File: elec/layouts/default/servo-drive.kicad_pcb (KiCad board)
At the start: 4 copper layers, 42.3 x 42.3 mm, 109 parts

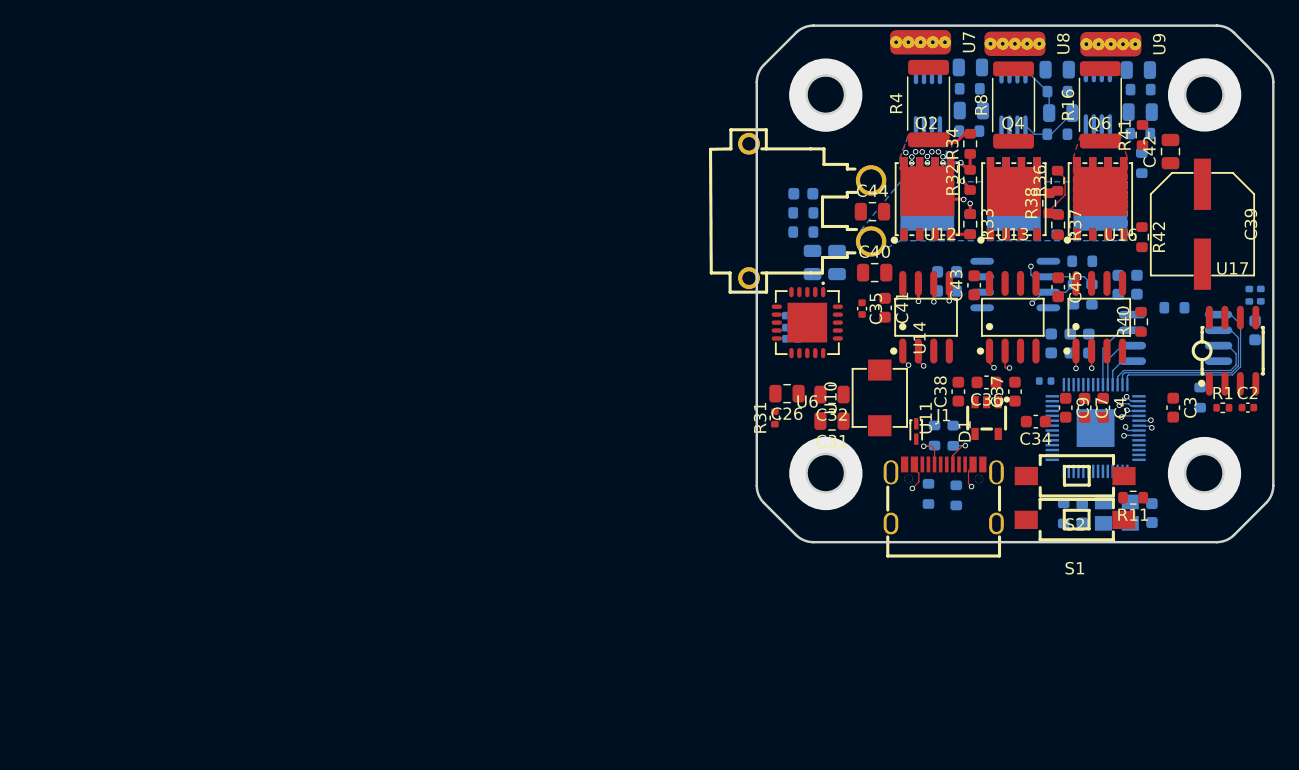
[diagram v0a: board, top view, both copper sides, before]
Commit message: layout complete
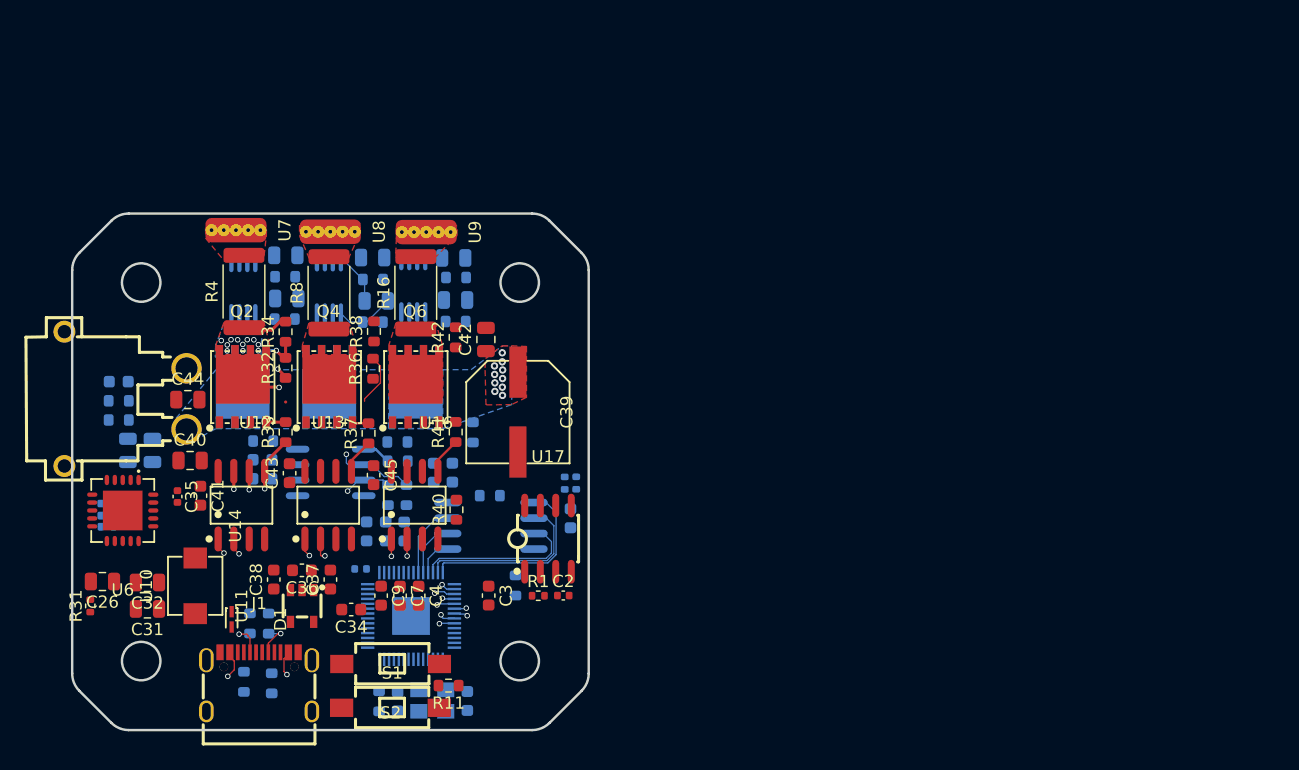
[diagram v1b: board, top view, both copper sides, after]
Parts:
- moved R41 61.3 mm to (162.2, 95.8)
- moved R35 60.6 mm to (146.5, 96.5), turned to 180 degrees
- moved R43 59.1 mm to (163.6, 95.8)
- moved R37 59.0 mm to (155.1, 95.9), turned to 90 degrees
- moved R33 58.6 mm to (148.3, 95.8), turned to 90 degrees
- moved R45 58.5 mm to (158.2, 100.9)
- moved R46 58.5 mm to (156.7, 100.9)
- moved R44 58.4 mm to (157.5, 98.1)
- moved C16 58.1 mm to (148.4, 84.8)
- moved C18 58.1 mm to (155.7, 85.0)
- moved C28 58.1 mm to (137.4, 97.3)
- moved C29 58.1 mm to (135.4, 97.3)
- moved C36 58.1 mm to (149.6, 107.1)
- moved C42 58.1 mm to (164.7, 88.2)
- moved C43 58.1 mm to (148.6, 99.1)
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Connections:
- J1 pad B5: servo_drive.ato/ServoDrive.gnd -> servo_drive.ato/ServoDrive.usb/cc2
- R20 pad 1: servo_drive.ato/ServoDrive/r_cc2/p1.ea763f -> servo_drive.ato/ServoDrive.usb/cc2
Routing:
- net servo_drive.ato/ServoDrive/power_stage/half_bridge_c.gate_driver/lvg: track 0.00 -> 3.00 mm
- net servo_drive.ato/ServoDrive/power_stage/half_bridge_b.gate_driver/lvg: track 0.00 -> 2.87 mm
- net servo_drive.ato/ServoDrive/position_sensor.sensor/PGO: track 0.00 -> 2.36 mm
- net servo_drive.ato/ServoDrive/power_stage/half_bridge_a.gate_driver/lvg: track 11.0 -> 13.2 mm, vias 2 -> 1
- net servo_drive.ato/ServoDrive/power_stage/half_bridge_c.ls_fet/gate: track 0.00 -> 1.38 mm
- net servo_drive.ato/ServoDrive/power_stage/half_bridge_b.ls_fet/gate: track 0.00 -> 1.34 mm
- net (no net): vias 17 -> 23
- added copper zone on F.Cu, net servo_drive.ato/ServoDrive.power_stage/out_b
- added copper zone on F.Cu, net servo_drive.ato/ServoDrive.power_stage/out_c
- added copper zone on F.Cu, net servo_drive.ato/ServoDrive.vbatt
